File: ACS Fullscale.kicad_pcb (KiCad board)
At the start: 2 copper layers, 151 x 151 mm, 61 parts, among them J1 Pulse-20, J2 Conn_01x02, J3 Conn_02x07_Odd_Even, J4 Conn_01x03, J5 Conn_01x03, J6 Conn_01x05, J7 THD-02-R, J8 Micro_SD_Card_Det, J9 Conn_01x02, Q1 Q_NPN_BEC, U1 SN65HVD230, U10 BNO086, U11 R-78E5.0-1.0, U12 TPD4EUSB30, U13 RT9742GGJ5, U14 MagJack-A70-112-331N126, U2 MS5611-01BA, U3 TPD4EUSB30, U4 Teensy4.1, U5 TPS62202DBV, U6 BHI360, U7 TXS0108EPW, U8 BMP581, U9 BME280, Y1 32.768k

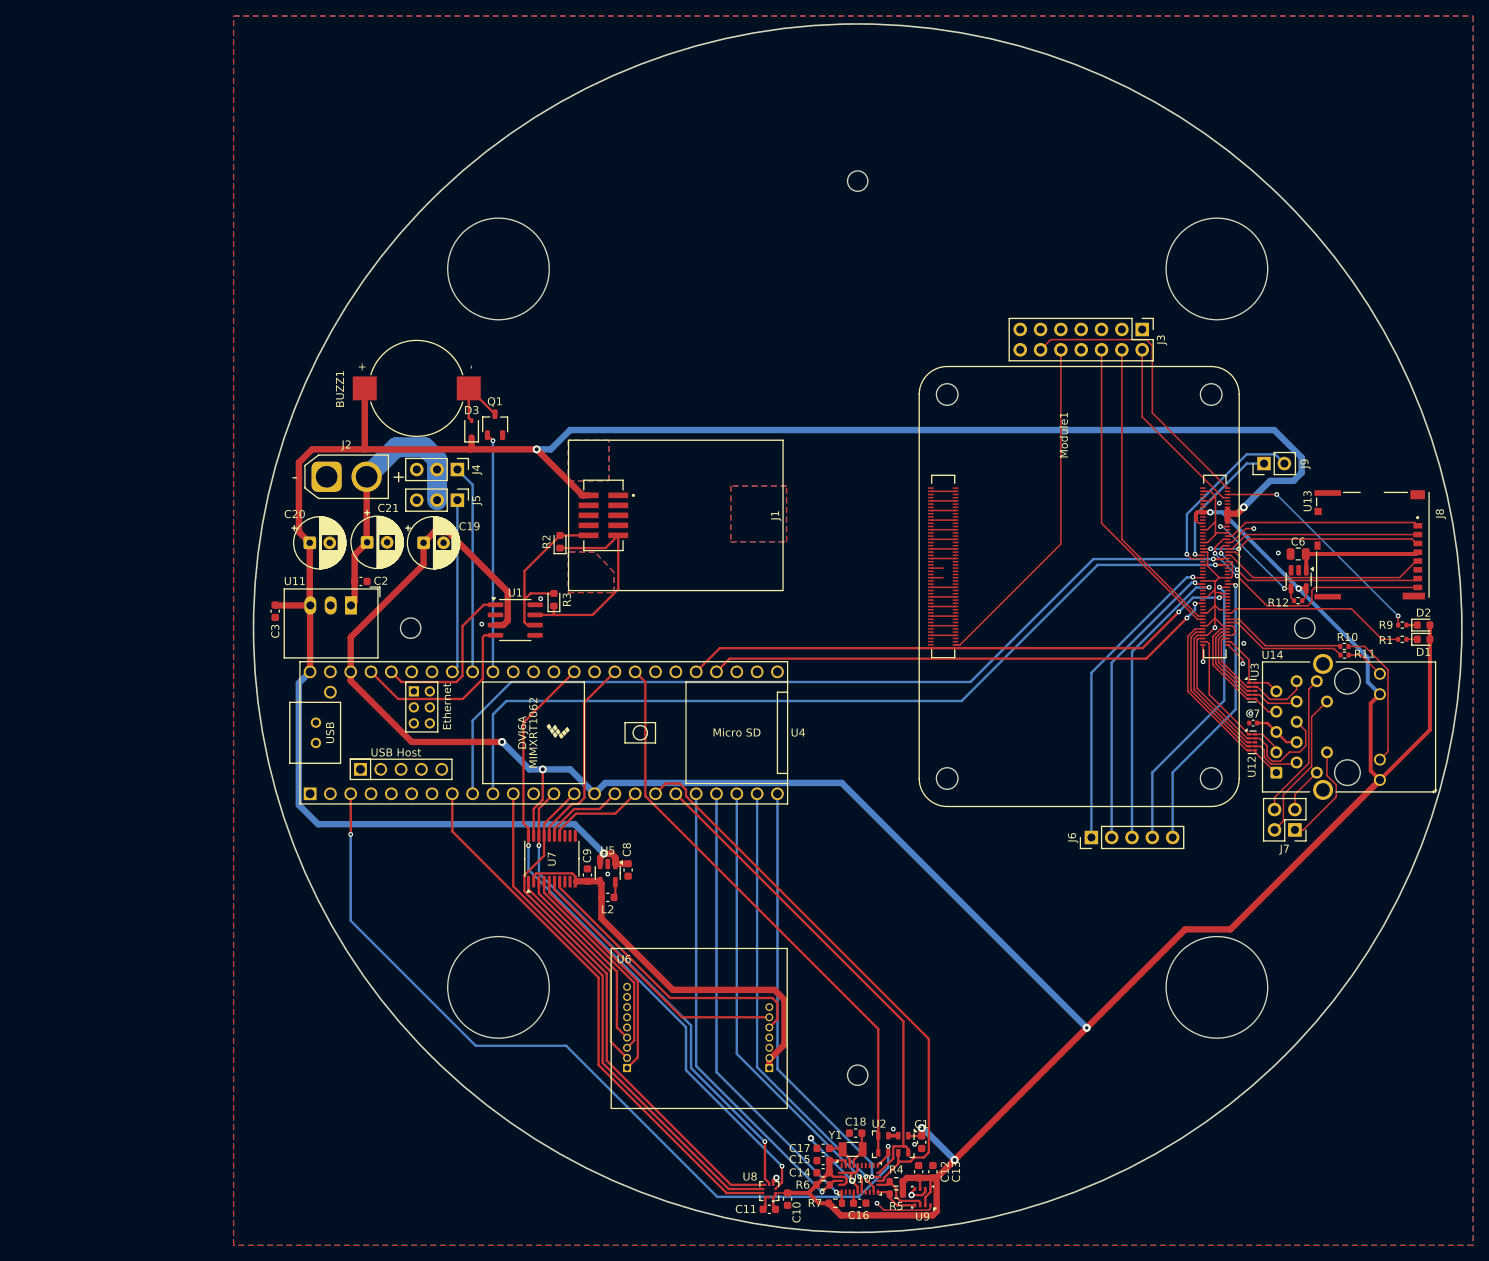
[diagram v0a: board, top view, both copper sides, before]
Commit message: lots
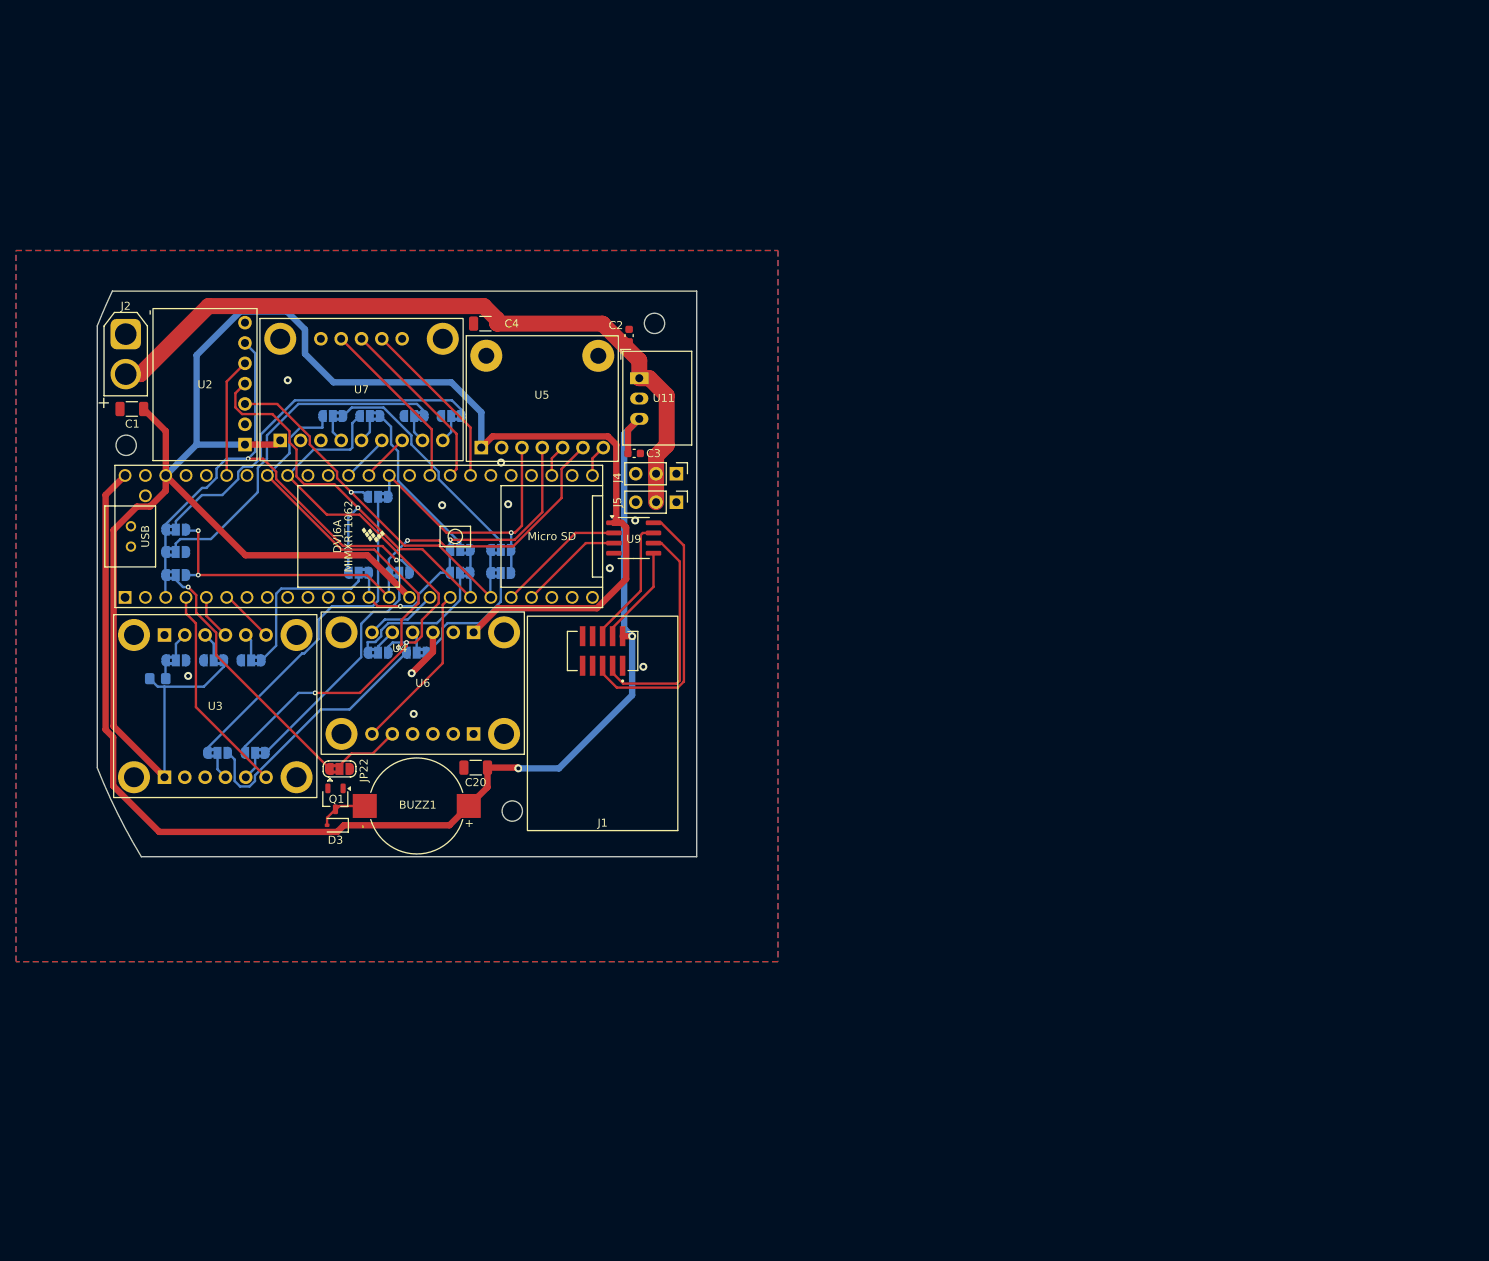
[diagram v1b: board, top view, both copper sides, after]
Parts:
- removed C10, C11, C12, C13, C14, C15, C16: 100nF, Capacitor_SMD:C_0603_1608Metric
- removed C17, C18: 22pF, Capacitor_SMD:C_0603_1608Metric
- removed C19, C21: 100uF, Capacitor_THT:CP_Radial_D6.3mm_P2.50mm
- removed C6: 10u, Capacitor_SMD:C_0805_2012Metric
- removed C7: 100n, Capacitor_SMD:C_0402_1005Metric
- removed C8: 4.7uF, Capacitor_SMD:C_0603_1608Metric
- removed C9: 10uF, Capacitor_SMD:C_0603_1608Metric
- removed D1: LED Green, LED_SMD:LED_0603_1608Metric
- removed D2: LED Red, LED_SMD:LED_0603_1608Metric
- removed J3: Conn_02x07_Odd_Even, Connector_PinHeader_2.54mm:PinHeader_2x07_P2.54mm_Vertical
- removed J6: Conn_01x05, Connector_PinHeader_2.54mm:PinHeader_1x05_P2.54mm_Vertical
- removed J7: THD-02-R, Connector_PinHeader_2.54mm:PinHeader_2x02_P2.54mm_Vertical
- removed J8: Micro_SD_Card_Det, CM5IO:SDCARD_MOLEX_503398-1892
- removed J9: Conn_01x02, Connector_PinHeader_2.54mm:PinHeader_1x02_P2.54mm_Vertical
- removed L2: 10uH, Inductor_SMD:L_0603_1608Metric
- removed Module1: ComputeModule5-CM5, CM5IO:Raspberry-Pi-5-Compute-Module
- removed R10, R11: 470R, Resistor_SMD:R_0402_1005Metric
- removed R12: 10K 1%, Resistor_SMD:R_0402_1005Metric
- removed R2, R3: 120, LED_SMD:LED_0603_1608Metric
- removed R4, R5: 4.7k, Resistor_SMD:R_0603_1608Metric
- removed R6, R7: 10k, Resistor_SMD:R_0603_1608Metric
- removed R9: 1k, Resistor_SMD:R_0402_1005Metric
- removed U1: SN65HVD230, Package_SO:SOIC-8_3.9x4.9mm_P1.27mm
- removed U10: BNO086, Package_LGA:LGA-28_5.2x3.8mm_P0.5mm
- removed U12: TPD4EUSB30, Package_SON:USON-10_2.5x1.0mm_P0.5mm
- removed U13: RT9742GGJ5, Package_TO_SOT_SMD:SOT-23-5
- removed U14: MagJack-A70-112-331N126, CM5IO:TRJG0926HENL
- removed U8: BMP581, ACS_Footprint_Library:QFN10_BMP581_BOS
- removed Y1: 32.768k, Crystal:Crystal_SMD_3215-2Pin_3.2x1.5mm
- added C4: 100uF, Capacitor_SMD:C_1206_3216Metric, F.Cu at (105.9, 61.0)
- added JP1: BNO_DI, Jumper:SolderJumper-3_P1.3mm_Bridged2Bar12_RoundedPad1.0x1.5mm, B.Cu at (76.6, 103.1)
- added JP10: LSM_SDOAG, Jumper:SolderJumper-3_P1.3mm_Bridged2Bar12_RoundedPad1.0x1.5mm, B.Cu at (97.0, 72.5)
- added JP11: LSM_SDOM, Jumper:SolderJumper-3_P1.3mm_Bridged2Bar12_RoundedPad1.0x1.5mm, B.Cu at (101.6, 72.5)
- added JP12: BNO_MOSI, Jumper:SolderJumper-3_P1.3mm_Bridged2Bar12_RoundedPad1.0x1.5mm, B.Cu at (90.0, 92.1)
- added JP13: BNO_SCK, Jumper:SolderJumper-3_P1.3mm_Bridged2Bar12_RoundedPad1.0x1.5mm, B.Cu at (92.4, 82.6)
- added JP14: BNO_MISO, Jumper:SolderJumper-3_P1.3mm_Bridged2Bar12_RoundedPad1.0x1.5mm, B.Cu at (95.1, 92.1)
- added JP15: LSM_SCK, Jumper:SolderJumper-3_P1.3mm_Bridged2Bar12_RoundedPad1.0x1.5mm, B.Cu at (107.8, 89.3)
- added JP16: LSM_MOSI, Jumper:SolderJumper-3_P1.3mm_Bridged2Bar12_RoundedPad1.0x1.5mm, B.Cu at (102.7, 89.3)
- added JP17: LSMAG_MISO, Jumper:SolderJumper-3_P1.3mm_Bridged2Bar12_RoundedPad1.0x1.5mm, B.Cu at (67.2, 92.4)
- added JP18: ICM_SCL, Jumper:SolderJumper-3_P1.3mm_Bridged2Bar12_RoundedPad1.0x1.5mm, B.Cu at (97.3, 102.1)
- added JP19: LSMAG_MISO, Jumper:SolderJumper-3_P1.3mm_Bridged2Bar12_RoundedPad1.0x1.5mm, B.Cu at (67.2, 89.5)
- added JP2: BNO_SCL, Jumper:SolderJumper-3_P1.3mm_Bridged2Bar12_RoundedPad1.0x1.5mm, B.Cu at (72.4, 114.6)
- added JP20: LSMM_MISO, Jumper:SolderJumper-3_P1.3mm_Bridged2Bar12_RoundedPad1.0x1.5mm, B.Cu at (67.2, 86.7)
- added JP21: ICM_SDA, Jumper:SolderJumper-3_P1.3mm_Bridged2Bar12_RoundedPad1.0x1.5mm, B.Cu at (92.4, 102.1)
- added JP22: ICM_SDO, Jumper:SolderJumper-3_P1.3mm_Bridged2Bar12_RoundedPad1.0x1.5mm, F.Cu at (87.6, 116.7)
- added JP3: BNO_SDA, Jumper:SolderJumper-3_P1.3mm_Bridged2Bar12_RoundedPad1.0x1.5mm, B.Cu at (77.1, 114.6)
- added JP4: BNO_P0, Jumper:SolderJumper-3_P1.3mm_Bridged2Bar12_RoundedPad1.0x1.5mm, B.Cu at (67.2, 103.1)
- added JP5: BNO_P1, Jumper:SolderJumper-3_P1.3mm_Bridged2Bar12_RoundedPad1.0x1.5mm, B.Cu at (71.9, 103.1)
- added JP6: LSM_SCL, Jumper:SolderJumper-3_P1.3mm_Bridged2Bar12_RoundedPad1.0x1.5mm, B.Cu at (86.8, 72.5)
- added JP7: LSM_SDA, Jumper:SolderJumper-3_P1.3mm_Bridged2Bar12_RoundedPad1.0x1.5mm, B.Cu at (91.4, 72.5)
- added JP8: LSM_SCK, Jumper:SolderJumper-3_P1.3mm_Bridged2Bar12_RoundedPad1.0x1.5mm, B.Cu at (107.8, 92.2)
- added JP9: LSM_MOSI, Jumper:SolderJumper-3_P1.3mm_Bridged2Bar12_RoundedPad1.0x1.5mm, B.Cu at (102.7, 92.1)
- C1: value 100nF -> 100uF; footprint Capacitor_SMD:C_0603_1608Metric -> Capacitor_SMD:C_1206_3216Metric
- C20: footprint Capacitor_THT:CP_Radial_D6.3mm_P2.50mm -> Capacitor_SMD:C_1206_3216Metric
- R1: value 1k -> 10k; footprint Resistor_SMD:R_0402_1005Metric -> Resistor_SMD:R_0805_2012Metric_Pad1.20x1.40mm_HandSolder; moved to B.Cu
- U2: value MS5611-01BA -> MS5611-01BA03; footprint Package_LGA:LGA-8_3x5mm_P1.25mm -> Sensor_Pressure:HiLetgo MS5611
- U3: value TPD4EUSB30 -> Adafruit_BNO086; footprint Package_SON:USON-10_2.5x1.0mm_P0.5mm -> Sensor_Motion:Adafruit BNO086
- U5: value TPS62202DBV -> BMP585; footprint Package_TO_SOT_SMD:SOT-23-5 -> Sensor_Pressure:DFRobot BMP585
- U6: value BHI360 -> ICM20948; footprint ACS_Footprint_Library:BHI360 Shuttle Board -> Sensor_Motion:Adafruit ICM20948
- U7: value TXS0108EPW -> LSM9DS1; footprint Package_SO:TSSOP-20_4.4x6.5mm_P0.65mm -> Sensor_Motion:Adafruit LSM9DS1
- U9: value BME280 -> LTC2851xS8; footprint Package_LGA:Bosch_LGA-8_2.5x2.5mm_P0.65mm_ClockwisePinNumbering -> Package_SO:SOIC-8_3.9x4.9mm_P1.27mm
- moved R1 155.6 mm to (64.9, 105.4)
- moved C1 134.7 mm to (61.7, 71.7), turned to 180 degrees
- moved U3 129.6 mm to (72.1, 108.8)
- moved U2 128.1 mm to (70.8, 68.6), turned to 90 degrees
- moved U9 90.0 mm to (124.4, 87.8), turned to 0 degrees
- moved U7 63.3 mm to (90.4, 69.2), turned to 0 degrees
- moved U5 60.1 mm to (113.0, 70.1), turned to 0 degrees
- moved U6 55.9 mm to (98.0, 105.9), turned to 180 degrees
- moved D3 52.4 mm to (87.1, 123.7), turned to 180 degrees
- moved BUZZ1 52.2 mm to (97.3, 121.3), turned to -90 degrees
- moved Q1 50.8 mm to (87.1, 120.4), turned to -90 degrees
- moved C3 49.0 mm to (124.5, 77.2), turned to 0 degrees
- moved U11 45.9 mm to (125.1, 67.8), turned to -90 degrees
- moved C2 45.5 mm to (123.8, 62.5), turned to 90 degrees
- moved C20 34.9 mm to (104.6, 116.5), turned to 180 degrees
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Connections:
- J1 pad 10: /CANL -> unconnected-(J1-CAN_L-Pad10)
- J1 pad 2: unconnected-(J1-PORT_A_Rx+-Pad2) -> /Rx+
- J1 pad 3: unconnected-(J1-PORT_A_Tx+-Pad3) -> /Tx+
- J1 pad 5: /CANH -> unconnected-(J1-CAN_H-Pad5)
- J1 pad 7: unconnected-(J1-PORT_A_RX--Pad7) -> /RX-
- J1 pad 8: unconnected-(J1-PORT_A_TX--Pad8) -> /TX-
- R1 pad 1: Net-(D1-K) -> /BNO_WAKE
- R1 pad 2: Net-(Module1A-LED_nACT) -> +3V3
- U2 pad 3: GND -> /SCK1
- U2 pad 4: /CS1 -> /MOSI1
- U2 pad 5: /CS1 -> /CS_MS
- U2 pad 7: /MOSI1 -> GND
- U3 pad 1: /CM5_GPIO ( Ethernet, GPIO, SDCARD)/TRD3_P -> +3V3
- U3 pad 10: /CM5_GPIO ( Ethernet, GPIO, SDCARD)/TRD3_P -> /BNO_RST
- U3 pad 2: /CM5_GPIO ( Ethernet, GPIO, SDCARD)/TRD3_N -> unconnected-(U3-3VO-Pad2)
- U3 pad 4: /CM5_GPIO ( Ethernet, GPIO, SDCARD)/TRD2_N -> /BNO_SCL
- U3 pad 5: /CM5_GPIO ( Ethernet, GPIO, SDCARD)/TRD2_P -> /BNO_SDA
- U3 pad 6: /CM5_GPIO ( Ethernet, GPIO, SDCARD)/TRD2_P -> /BNO_INT
- U3 pad 7: /CM5_GPIO ( Ethernet, GPIO, SDCARD)/TRD2_N -> unconnected-(U3-BT-Pad7)
- U3 pad 8: GND -> /BNO_P0
- U3 pad 9: /CM5_GPIO ( Ethernet, GPIO, SDCARD)/TRD3_N -> /BNO_P1
- U4 pad 11: /CS0 -> unconnected-(U4-9_OUT1C-Pad11)
- U4 pad 16: /INT2 -> /ICM_INT
- U4 pad 17: /RST2 -> /ICM_CS
- U4 pad 20: /BT3 -> /RX7
- U4 pad 21: /WAKE3 -> /TX7
- U4 pad 22: /RST3 -> unconnected-(U4-30_CRX3-Pad22)
- U4 pad 23: /INT3 -> unconnected-(U4-31_CTX3-Pad23)
- U4 pad 24: /CS3 -> unconnected-(U4-32_OUT1B-Pad24)
- U4 pad 25: unconnected-(U4-33_MCLK2-Pad25) -> /BMP_INT
- U4 pad 27: unconnected-(U4-35_TX8-Pad27) -> /BMP_CS
- U4 pad 28: /PWM2 -> unconnected-(U4-36_CS-Pad28)
- U4 pad 29: /PWM1 -> unconnected-(U4-37_CS-Pad29)
- U4 pad 31: unconnected-(U4-39_MISO1_OUT1A-Pad31) -> /LSM_INTM
- U4 pad 32: /CS1 -> /LSM_INT1
- U4 pad 33: /CS2 -> /LSM_INT2
- U4 pad 36: unconnected-(U4-14_A0_TX3_SPDIF_OUT-Pad36) -> /LSM_CSM
- U4 pad 37: unconnected-(U4-15_A1_RX3_SPDIF_IN-Pad37) -> /LSM_CSAG
- U4 pad 39: /Buzz -> unconnected-(U4-17_A3_TX4_SDA1-Pad39)
- U4 pad 4: unconnected-(U4-2_OUT2-Pad4) -> /BNO_INT
- U4 pad 40: /Motor1 -> /SDA
- U4 pad 41: /Motor2 -> /SCL
- U4 pad 43: unconnected-(U4-21_A7_RX5_BCLK1-Pad43) -> /CS_MS
- U4 pad 44: /CANTX -> /PWM2
- U4 pad 45: /CANRX -> /PWM1
- U4 pad 5: unconnected-(U4-3_LRCLK2-Pad5) -> /BNO_RST
- U4 pad 6: unconnected-(U4-4_BCLK2-Pad6) -> /BNO_CS
- U4 pad 8: /INT0 -> unconnected-(U4-6_OUT1D-Pad8)
- U5 pad 1: +5V -> +3V3
- U5 pad 3: +5V -> /SCK0
- U5 pad 4: +1V8 -> /MOSI0
- U5 pad 5: Net-(U5-SW) -> /BMP_CS
- U7 pad 1: /SCK_1V8 -> +3V3
- U7 pad 10: +1V8 -> unconnected-(U7-DEN-Pad10)
- U7 pad 11: GND -> /LSM_INT2
- U7 pad 12: unconnected-(U7-B8-Pad12) -> /LSM_INT1
- U7 pad 13: unconnected-(U7-B7-Pad13) -> /LSM_INTM
- U7 pad 14: /RST2 -> unconnected-(U7-DRDY-Pad14)
- U7 pad 2: +1V8 -> unconnected-(U7-3VO-Pad2)
- U7 pad 3: /MOSI_1V8 -> GND
- U7 pad 4: /MISO_1V8 -> /LSM_SCL
- U7 pad 5: /CS_1V8 -> /LSM_SDA
- U7 pad 6: /INT_1V8 -> /LSM_CSAG
- U7 pad 7: /RST_1V8 -> /LSM_CSM
- U7 pad 8: unconnected-(U7-A7-Pad8) -> /LSM_SDOAG
- U7 pad 9: unconnected-(U7-A8-Pad9) -> /LSM_SDOM
- U9 pad 1: GND -> +3V3
- U9 pad 2: +3V3 -> /RX7
- U9 pad 3: /BNO086/SDA -> /TX7
- U9 pad 4: /BNO086/SCL -> GND
- U9 pad 5: GND -> /RX-
- U9 pad 6: +3V3 -> /Rx+
- U9 pad 7: GND -> /TX-
- U9 pad 8: +3V3 -> /Tx+
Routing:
- net GND: track 161.3 -> 6.22 mm, vias 18 -> 10
- net +3V3: track 368.6 -> 247.5 mm, vias 7 -> 0
- net /RX2: track 111.9 -> 0.00 mm, vias 1 -> 0
- net /TX2: track 109.5 -> 0.00 mm, vias 1 -> 0
- net +5V: track 256.3 -> 157.9 mm, vias 3 -> 2
- net /SCL: track 0.00 -> 78.9 mm, vias 0 -> 1
- net /SDA: track 0.00 -> 77.1 mm, vias 0 -> 2
- net /CS1: track 72.7 -> 0.00 mm
- net /PWM1: track 70.3 -> 0.00 mm, vias 2 -> 0
- net /INT0: track 68.7 -> 0.00 mm
- net /CS0: track 64.9 -> 0.00 mm
- net /PWM2: track 64.8 -> 0.00 mm, vias 2 -> 0
- net /BT3: track 59.2 -> 0.00 mm, vias 1 -> 0
- net +BATT: track 33.0 -> 91.3 mm
- net /WAKE3: track 58.1 -> 0.00 mm, vias 1 -> 0
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- removed copper zone on B.Cu, net (none)
- removed copper zone on F.Cu, net (none)
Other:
- board size 151 x 151 mm -> 74.9 x 70.7 mm
